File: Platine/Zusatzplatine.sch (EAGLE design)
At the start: 25 parts

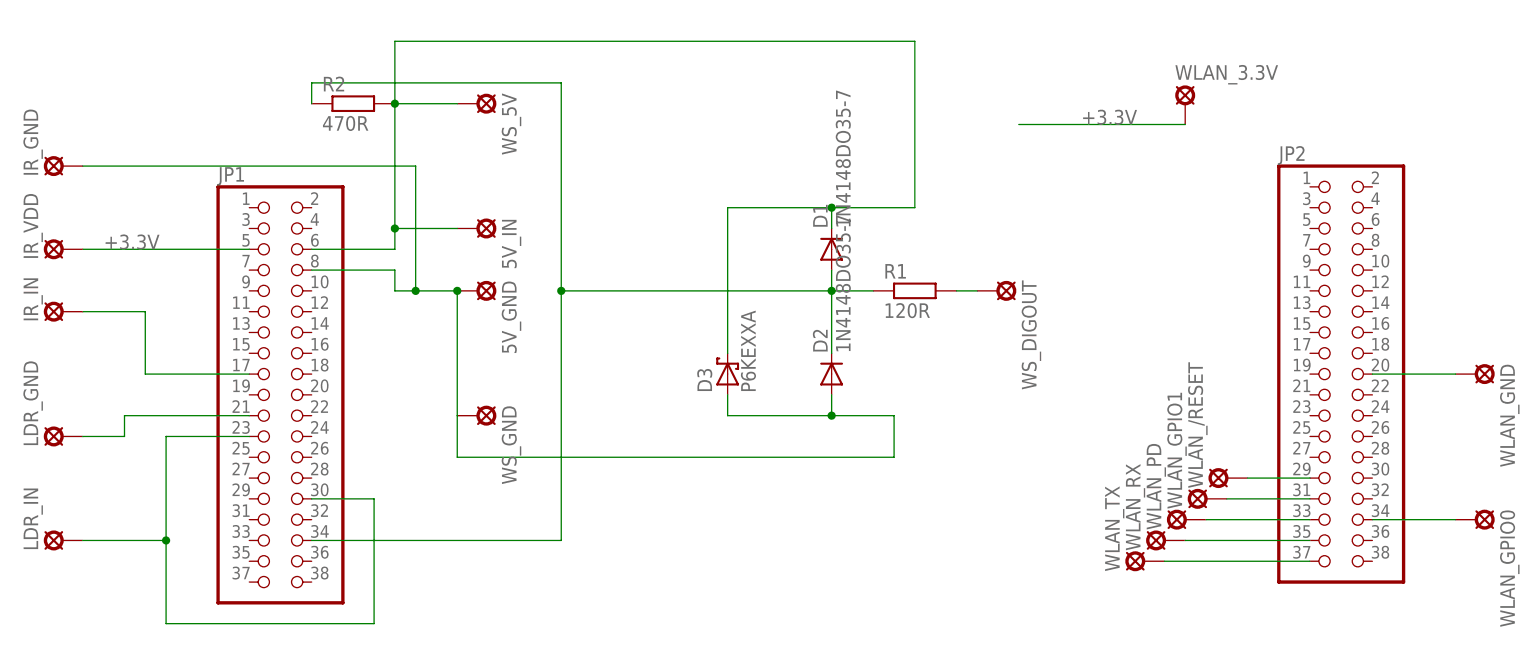
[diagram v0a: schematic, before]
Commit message: - Platine weiter
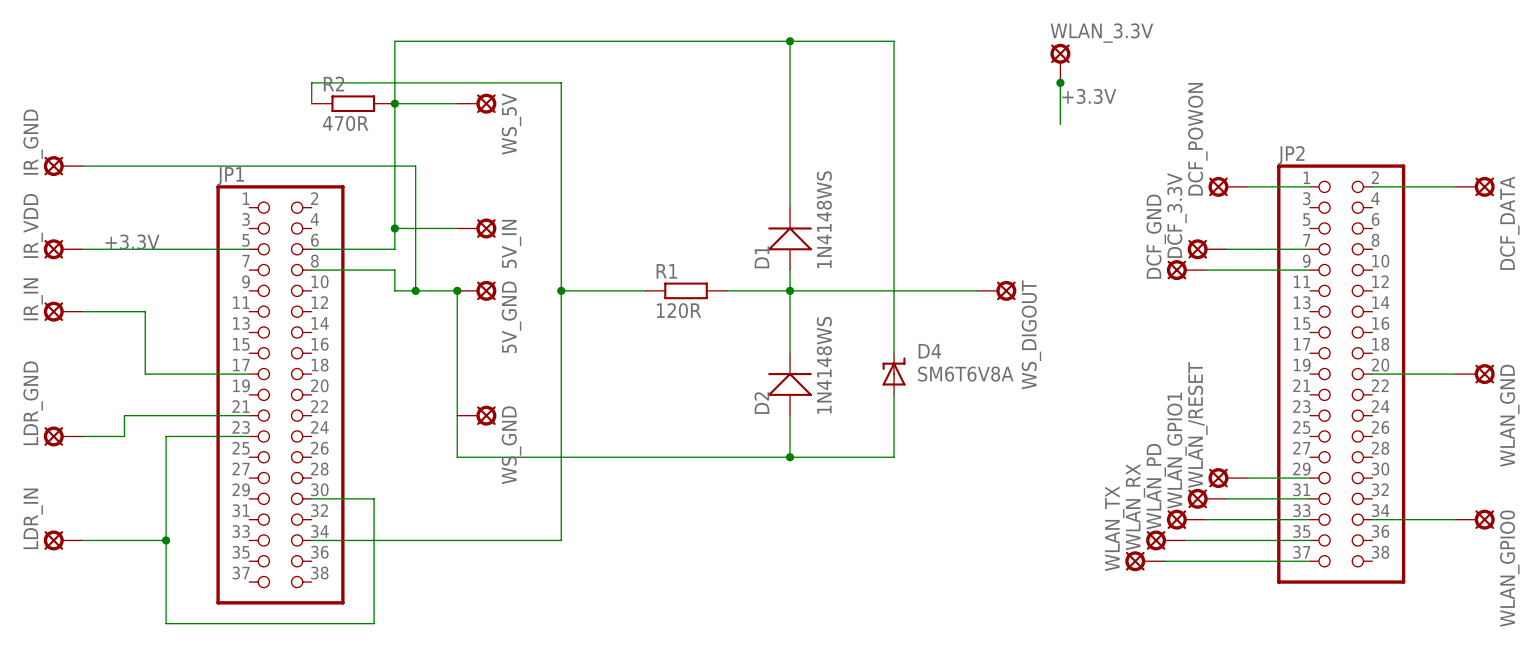
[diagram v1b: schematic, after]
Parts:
- removed D3: P6KEXXA, diode:P6KEXXA
- added D4: SM6T6V8A, diode:SUPPRESSOR-SMBG
- added DCF_3.3V, DCF_DATA, DCF_GND, DCF_POWON: SE14, solpad:SE14
- D1, D2: value 1N4148DO35-7 -> 1N4148WS; device diode:1N4148DO35-7 -> Diodes:1N4148WS
- R1, R2: device rcl:R-EU_0309/12 -> rcl:R-EU_R1206
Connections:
- removed net N$9: D2.A, D3.A
- new net N$17: DCF_GND.MP, JP2.9
- new net N$18: DCF_3.3V.MP, JP2.7
- new net N$19: DCF_POWON.MP, JP2.1
- new net N$20: DCF_DATA.MP, JP2.2
- net +3.3V: now also WLAN_3.3V.MP
- net N$10: now also D1.1, D4.C; no longer D1.C, D3.C
- net N$4: now also D2.0, D4.A
- net N$7: no longer D1.A, D2.C
- net N$8: now also D1.0, D2.1
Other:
- moved on the sheet: D1, D2, R1, WLAN_3.3V

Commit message: - Platine Fehler behoben
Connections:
- removed net N$5: 5V_IN.MP, JP1.6, R2.2, WS_5V.MP
- net N$10: now also 5V_IN.MP, JP1.6, R2.2, WS_5V.MP
